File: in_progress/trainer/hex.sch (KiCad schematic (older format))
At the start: 63 parts

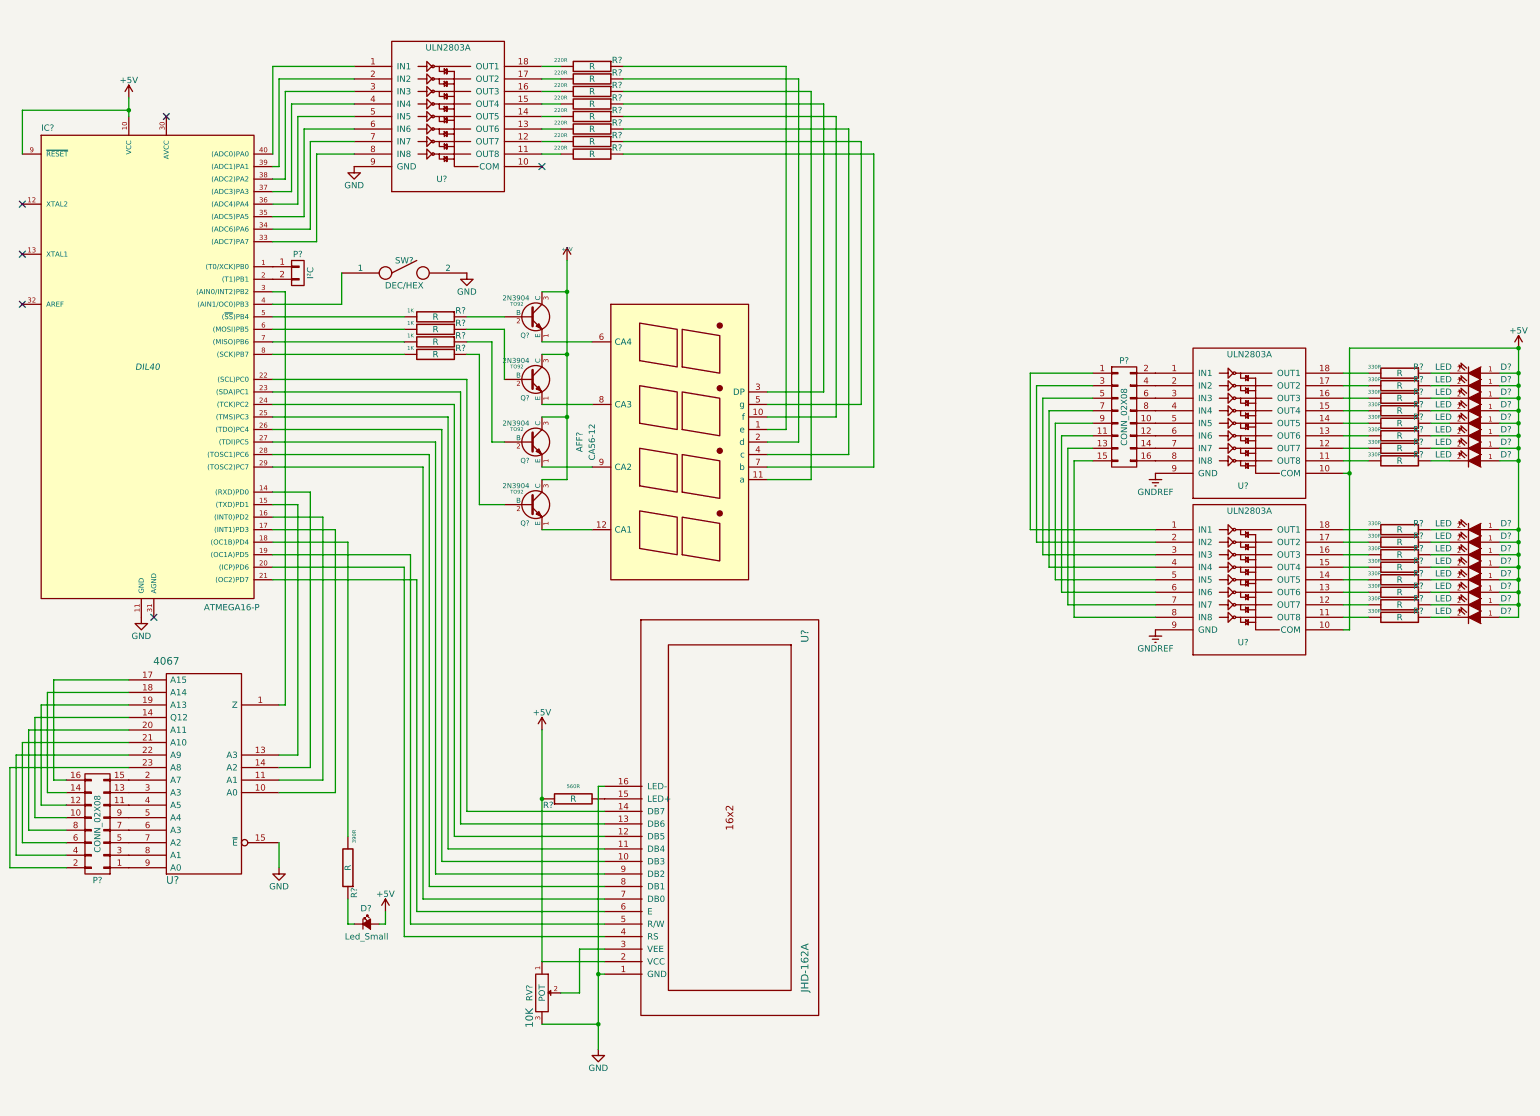
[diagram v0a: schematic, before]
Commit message: .
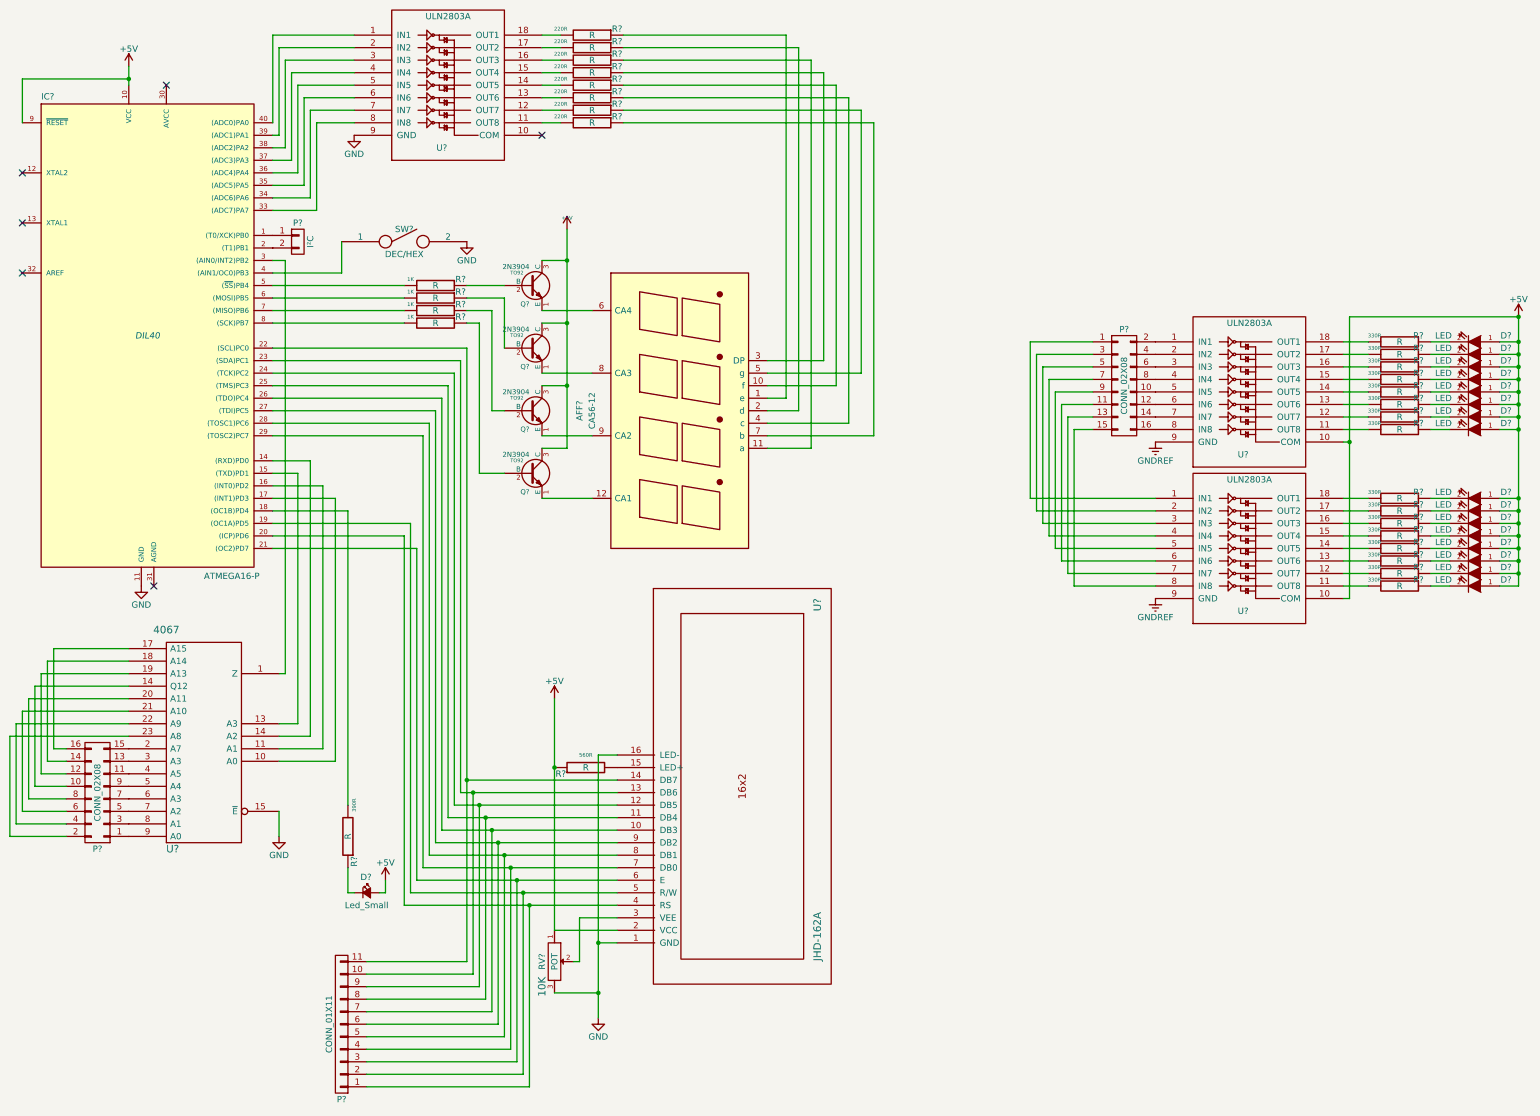
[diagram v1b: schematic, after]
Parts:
- added P?: CONN_01X11, symbol CONN_01X11
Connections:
- net at IC?.19 ((OC1A)PD5), U?.5 (R/W): now also P?.2 (P2)
- net at IC?.20 ((ICP)PD6), U?.4 (RS): now also P?.1 (P1)
- net at IC?.21 ((OC2)PD7), U?.6 (E): now also P?.3 (P3)
- net at IC?.22 ((SCL)PC0), U?.14 (DB7): now also P?.11 (P11)
- net at IC?.23 ((SDA)PC1), U?.13 (DB6): now also P?.10 (P10)
- net at IC?.24 ((TCK)PC2), U?.12 (DB5): now also P?.9 (P9)
- net at IC?.25 ((TMS)PC3), U?.11 (DB4): now also P?.8 (P8)
- net at IC?.26 ((TDO)PC4), U?.10 (DB3): now also P?.7 (P7)
- net at IC?.27 ((TDI)PC5), U?.9 (DB2): now also P?.6 (P6)
- net at IC?.28 ((TOSC1)PC6), U?.8 (DB1): now also P?.5 (P5)
- net at IC?.29 ((TOSC2)PC7), U?.7 (DB0): now also P?.4 (P4)
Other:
- moved on the sheet: AFF?, D?, IC?, P?, Q?, R?, RV?, SW?, U?
